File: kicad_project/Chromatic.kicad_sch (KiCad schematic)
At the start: 159 parts, among them J1 J1, J2 J2, U1 ESP32-S3

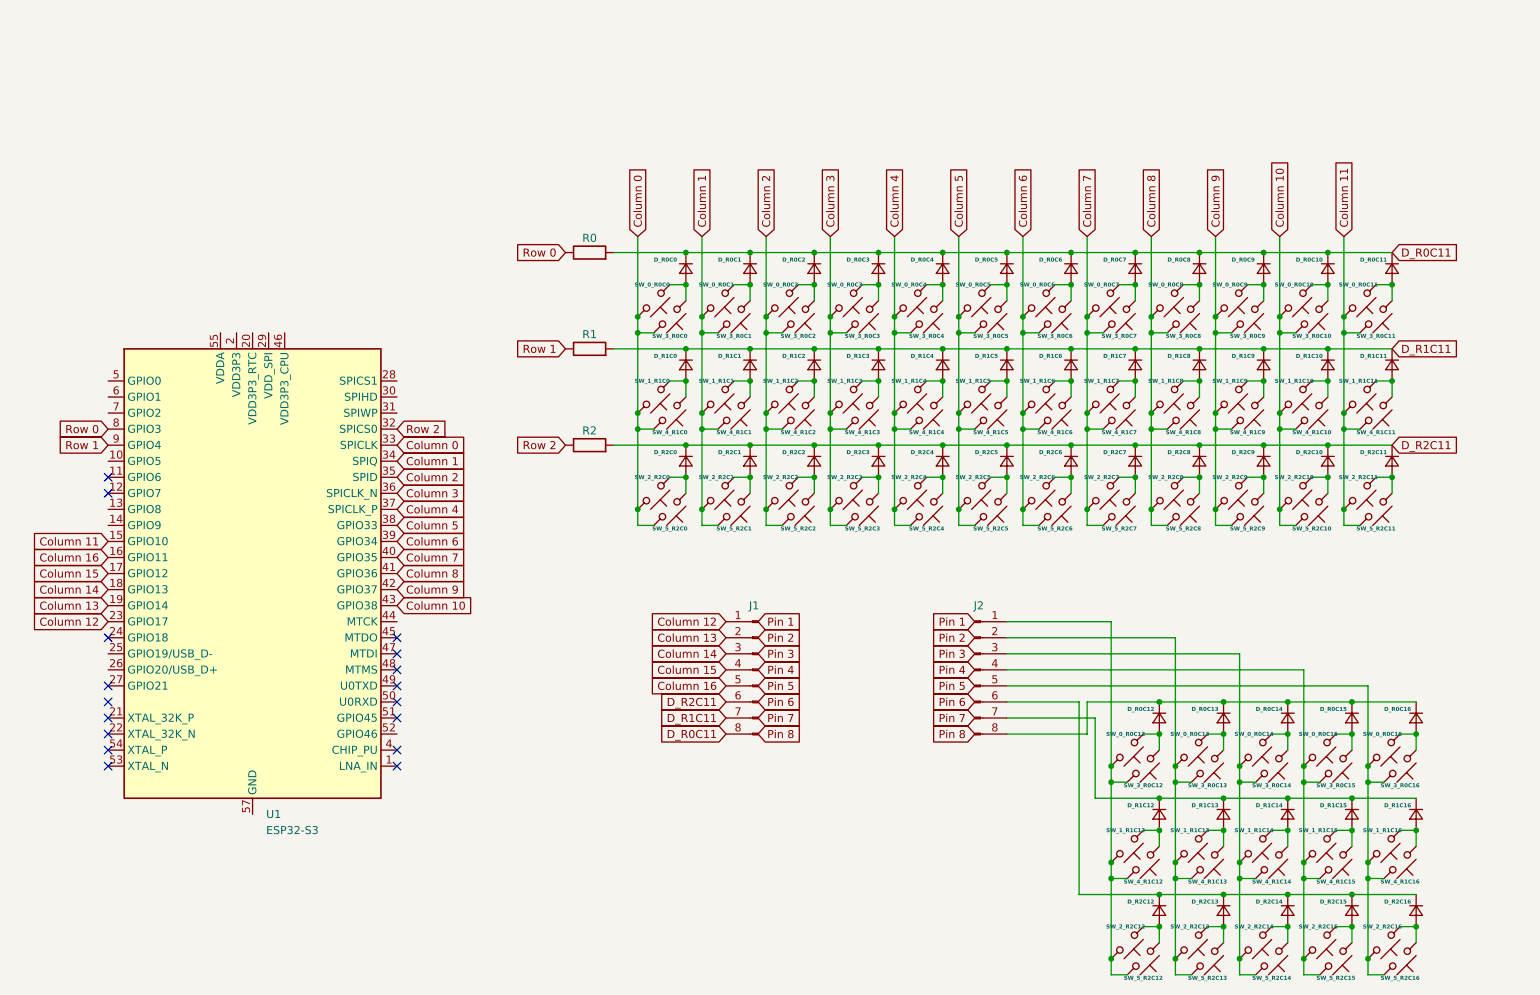
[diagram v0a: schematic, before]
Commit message: arrumado pcb e footprint
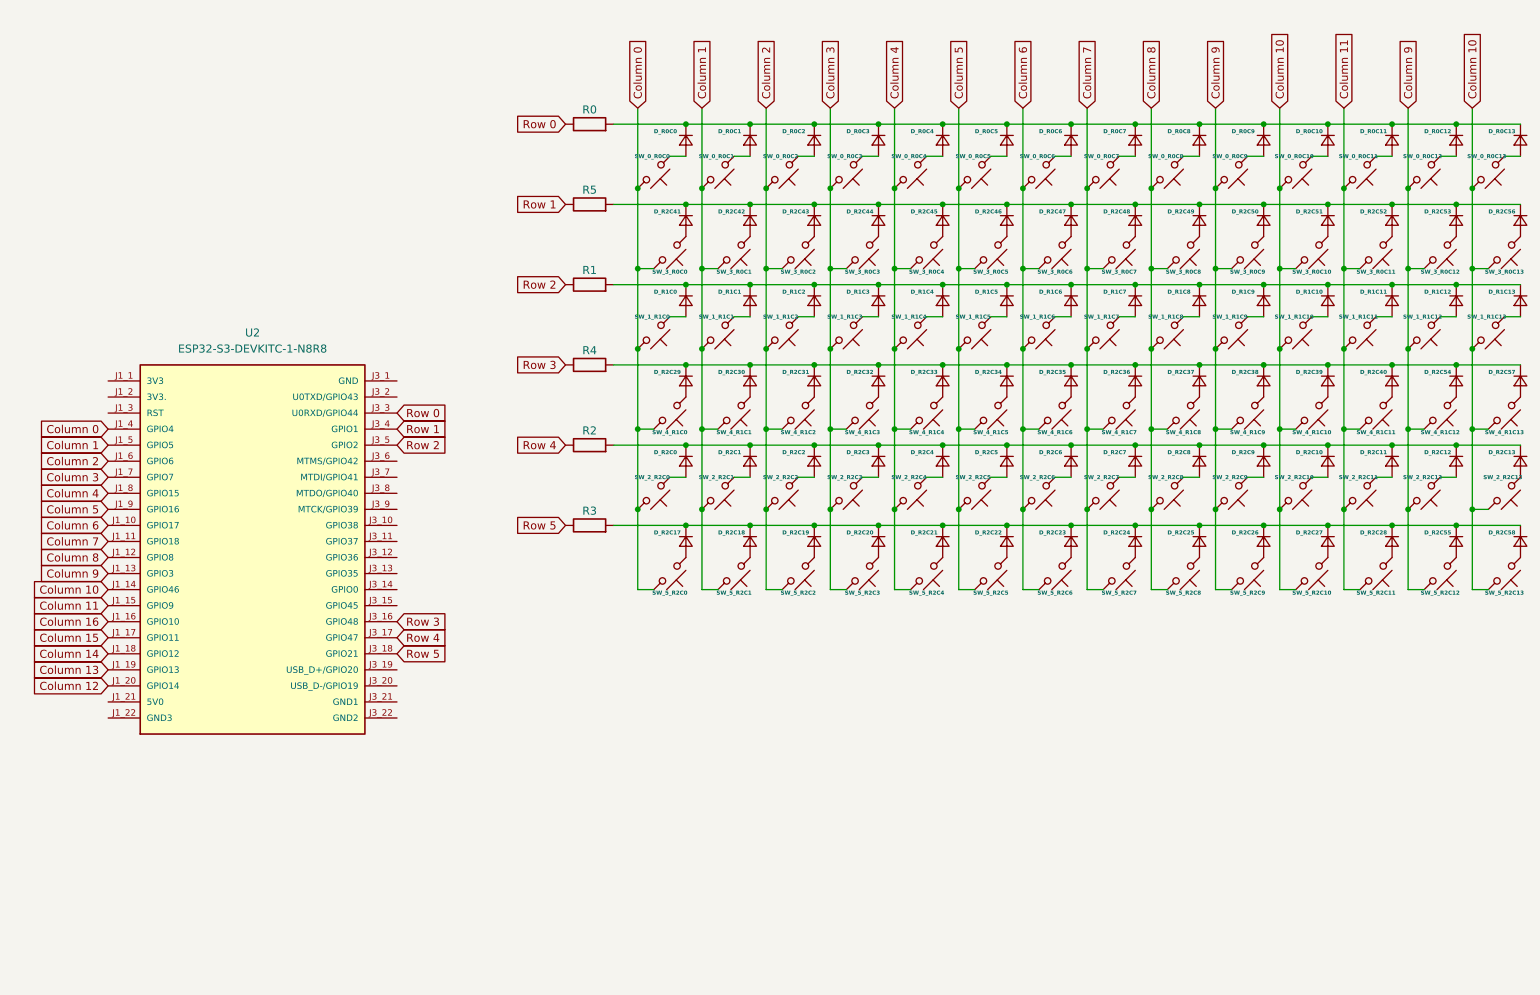
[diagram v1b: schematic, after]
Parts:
- removed D_R0C14, D_R0C15, D_R0C16, D_R1C14, D_R1C15, D_R1C16, D_R2C14, D_R2C15, D_R2C16: (no value), ScottoKeebs_Components:Diode_DO-35, symbol ScottoKeebs:Placeholder_Diode
- removed J1: J1, Connector_PinHeader_2.54mm:PinHeader_1x08_P2.54mm_Vertical, symbol Connector:Conn_01x08_Pin
- removed J2: J2, Connector_PinHeader_2.54mm:PinHeader_1x08_P2.54mm_Vertical, symbol Connector:Conn_01x08_Pin
- removed SW_0_R0C14, SW_0_R0C15, SW_0_R0C16, SW_1_R1C14, SW_1_R1C15, SW_1_R1C16, SW_2_R2C14, SW_2_R2C15, SW_2_R2C16, SW_3_R0C14, SW_3_R0C15, SW_3_R0C16, SW_4_R1C14, SW_4_R1C15, SW_4_R1C16, SW_5_R2C14, SW_5_R2C15, SW_5_R2C16: Keyswitch, ScottoKeebs_Hotswap:Hotswap_MX_1.00u, symbol ScottoKeebs:Placeholder_Keyswitch
- removed U1: ESP32-S3, Module:XCVR_ESP32-S3-DEVKIT-LIPO, symbol MCU_Espressif:ESP32-S3
- added D_R2C17, D_R2C18, D_R2C19, D_R2C20, D_R2C21, D_R2C22, D_R2C23, D_R2C24, D_R2C25, D_R2C26, D_R2C27, D_R2C28, D_R2C29, D_R2C30, D_R2C31, D_R2C32, D_R2C33, D_R2C34, D_R2C35, D_R2C36, D_R2C37, D_R2C38, D_R2C39, D_R2C40, D_R2C41, D_R2C42, D_R2C43, D_R2C44, D_R2C45, D_R2C46, D_R2C47, D_R2C48, D_R2C49, D_R2C50, D_R2C51, D_R2C52, D_R2C53, D_R2C54, D_R2C55, D_R2C56, D_R2C57, D_R2C58: (no value), ScottoKeebs_Components:Diode_DO-35, symbol ScottoKeebs:Placeholder_Diode
- added R3, R4, R5: Resistor, Resistor_THT:R_Axial_DIN0207_L6.3mm_D2.5mm_P7.62mm_Horizontal, symbol ScottoKeebs:Placeholder_Resistor
- added U2: ESP32-S3-DEVKITC-1-N8R8, RF_Module:ESP32-S3-DEVKITC-1-N8R8, symbol ESP32-S3-DEVKITC-1-N8R8:ESP32-S3-DEVKITC-1-N8R8
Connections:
- net D_R0C11 is gone; now on an unnamed net: D_R0C0.1 (K), D_R0C1.1 (K), D_R0C10.1 (K), D_R0C11.1 (K), D_R0C2.1 (K), D_R0C3.1 (K), D_R0C4.1 (K), D_R0C5.1 (K), D_R0C6.1 (K), D_R0C7.1 (K), D_R0C8.1 (K), D_R0C9.1 (K), R0.2
- net D_R1C11 is gone; now on an unnamed net: D_R1C0.1 (K), D_R1C1.1 (K), D_R1C10.1 (K), D_R1C11.1 (K), D_R1C2.1 (K), D_R1C3.1 (K), D_R1C4.1 (K), D_R1C5.1 (K), D_R1C6.1 (K), D_R1C7.1 (K), D_R1C8.1 (K), D_R1C9.1 (K), R1.2
- net D_R2C11 is gone; now on an unnamed net: D_R2C0.1 (K), D_R2C1.1 (K), D_R2C10.1 (K), D_R2C11.1 (K), D_R2C2.1 (K), D_R2C3.1 (K), D_R2C4.1 (K), D_R2C5.1 (K), D_R2C6.1 (K), D_R2C7.1 (K), D_R2C8.1 (K), D_R2C9.1 (K), R2.2
- net Column 0: now also U2.J1_4 (GPIO4)
- net Column 1: now also U2.J1_5 (GPIO5)
- net Column 10: now also SW_0_R0C13.1, SW_1_R1C13.1, SW_2_R2C13.1, SW_3_R0C13.1, SW_4_R1C13.1, SW_5_R2C13.1, U2.J1_14 (GPIO46)
- net Column 11: now also U2.J1_15 (GPIO9)
- net Column 12: now also U2.J1_20 (GPIO14)
- net Column 13: now also U2.J1_19 (GPIO13)
- net Column 14: now also U2.J1_18 (GPIO12)
- net Column 15: now also U2.J1_17 (GPIO11)
- net Column 16: now also U2.J1_16 (GPIO10)
- net Column 2: now also U2.J1_6 (GPIO6)
- net Column 3: now also U2.J1_7 (GPIO7)
- net Column 4: now also U2.J1_8 (GPIO15)
- net Column 5: now also U2.J1_9 (GPIO16)
- net Column 6: now also U2.J1_10 (GPIO17)
- net Column 7: now also U2.J1_11 (GPIO18)
- net Column 8: now also U2.J1_12 (GPIO8)
- net Column 9: now also SW_0_R0C12.1, SW_1_R1C12.1, SW_2_R2C12.1, SW_3_R0C12.1, SW_4_R1C12.1, SW_5_R2C12.1, U2.J1_13 (GPIO3)
- net Row 0: now also U2.J3_3 (U0RXD/GPIO44)
- net Row 1: now also R5.1, U2.J3_4 (GPIO1); no longer R1.1
- net Row 2: now also R1.1, U2.J3_5 (GPIO2); no longer R2.1
- net at D_R1C7.2 (A), SW_1_R1C7.2: no longer SW_4_R1C7.2
- net at D_R0C3.2 (A), SW_0_R0C3.2: no longer SW_3_R0C3.2
- net at D_R2C4.2 (A), SW_2_R2C4.2: no longer SW_5_R2C4.2
- net at D_R1C0.2 (A), SW_1_R1C0.2: no longer SW_4_R1C0.2
- net at D_R2C2.2 (A), SW_2_R2C2.2: no longer SW_5_R2C2.2
- net at D_R0C1.2 (A), SW_0_R0C1.2: no longer SW_3_R0C1.2
- net at D_R1C8.2 (A), SW_1_R1C8.2: no longer SW_4_R1C8.2
- net at D_R1C13.2 (A), SW_1_R1C13.2: no longer SW_4_R1C13.2
- net at D_R2C1.2 (A), SW_2_R2C1.2: no longer SW_5_R2C1.2
- net at D_R2C6.2 (A), SW_2_R2C6.2: no longer SW_5_R2C6.2
- net at D_R2C5.2 (A), SW_2_R2C5.2: no longer SW_5_R2C5.2
- net at D_R1C3.2 (A), SW_1_R1C3.2: no longer SW_4_R1C3.2
- net at D_R2C0.2 (A), SW_2_R2C0.2: no longer SW_5_R2C0.2
- net at D_R1C4.2 (A), SW_1_R1C4.2: no longer SW_4_R1C4.2
- net at D_R2C13.2 (A), SW_2_R2C13.2: no longer SW_5_R2C13.2
- net at D_R0C7.2 (A), SW_0_R0C7.2: no longer SW_3_R0C7.2
- net at D_R0C0.2 (A), SW_0_R0C0.2: no longer SW_3_R0C0.2
- net at D_R1C9.2 (A), SW_1_R1C9.2: no longer SW_4_R1C9.2
- net at D_R1C1.2 (A), SW_1_R1C1.2: no longer SW_4_R1C1.2
- net at D_R0C2.2 (A), SW_0_R0C2.2: no longer SW_3_R0C2.2
- net at D_R1C6.2 (A), SW_1_R1C6.2: no longer SW_4_R1C6.2
- net at D_R0C13.2 (A), SW_0_R0C13.2: no longer SW_3_R0C13.2
- net at D_R0C6.2 (A), SW_0_R0C6.2: no longer SW_3_R0C6.2
- net at D_R0C11.2 (A), SW_0_R0C11.2: no longer SW_3_R0C11.2
- net at D_R1C11.2 (A), SW_1_R1C11.2: no longer SW_4_R1C11.2
- net at D_R1C2.2 (A), SW_1_R1C2.2: no longer SW_4_R1C2.2
- net at D_R2C9.2 (A), SW_2_R2C9.2: no longer SW_5_R2C9.2
- net at D_R2C10.2 (A), SW_2_R2C10.2: no longer SW_5_R2C10.2
- net at D_R2C3.2 (A), SW_2_R2C3.2: no longer SW_5_R2C3.2
- net at D_R1C5.2 (A), SW_1_R1C5.2: no longer SW_4_R1C5.2
- net at D_R0C8.2 (A), SW_0_R0C8.2: no longer SW_3_R0C8.2
- net at D_R2C8.2 (A), SW_2_R2C8.2: no longer SW_5_R2C8.2
- net at D_R0C5.2 (A), SW_0_R0C5.2: no longer SW_3_R0C5.2
- net at D_R0C4.2 (A), SW_0_R0C4.2: no longer SW_3_R0C4.2
- net at D_R2C12.2 (A), SW_2_R2C12.2: no longer SW_5_R2C12.2
- net at D_R2C7.2 (A), SW_2_R2C7.2: no longer SW_5_R2C7.2
- net at D_R0C9.2 (A), SW_0_R0C9.2: no longer SW_3_R0C9.2
- net at D_R0C10.2 (A), SW_0_R0C10.2: no longer SW_3_R0C10.2
- net at D_R2C11.2 (A), SW_2_R2C11.2: no longer SW_5_R2C11.2
- net at D_R1C10.2 (A), SW_1_R1C10.2: no longer SW_4_R1C10.2
- net at D_R1C12.2 (A), SW_1_R1C12.2: no longer SW_4_R1C12.2
- net at D_R0C12.2 (A), SW_0_R0C12.2: no longer SW_3_R0C12.2
- new net: D_R2C44.2 (A), SW_3_R0C3.2
- new net: D_R2C55.2 (A), SW_5_R2C12.2
- new net: D_R2C41.1 (K), D_R2C42.1 (K), D_R2C43.1 (K), D_R2C44.1 (K), D_R2C45.1 (K), D_R2C46.1 (K), D_R2C47.1 (K), D_R2C48.1 (K), D_R2C49.1 (K), D_R2C50.1 (K), D_R2C51.1 (K), D_R2C52.1 (K), D_R2C53.1 (K), D_R2C56.1 (K), R5.2
- new net: D_R2C53.2 (A), SW_3_R0C12.2
- new net: D_R2C17.1 (K), D_R2C18.1 (K), D_R2C19.1 (K), D_R2C20.1 (K), D_R2C21.1 (K), D_R2C22.1 (K), D_R2C23.1 (K), D_R2C24.1 (K), D_R2C25.1 (K), D_R2C26.1 (K), D_R2C27.1 (K), D_R2C28.1 (K), D_R2C55.1 (K), D_R2C58.1 (K), R3.2
- new net: D_R2C50.2 (A), SW_3_R0C9.2
- new net: D_R2C37.2 (A), SW_4_R1C8.2
- new net: D_R2C22.2 (A), SW_5_R2C5.2
- new net: D_R2C56.2 (A), SW_3_R0C13.2
- new net: D_R2C43.2 (A), SW_3_R0C2.2
- new net: D_R2C29.1 (K), D_R2C30.1 (K), D_R2C31.1 (K), D_R2C32.1 (K), D_R2C33.1 (K), D_R2C34.1 (K), D_R2C35.1 (K), D_R2C36.1 (K), D_R2C37.1 (K), D_R2C38.1 (K), D_R2C39.1 (K), D_R2C40.1 (K), D_R2C54.1 (K), D_R2C57.1 (K), R4.2
- new net: D_R2C33.2 (A), SW_4_R1C4.2
- new net: D_R2C38.2 (A), SW_4_R1C9.2
- new net: D_R2C36.2 (A), SW_4_R1C7.2
- new net: D_R2C41.2 (A), SW_3_R0C0.2
- new net: D_R2C23.2 (A), SW_5_R2C6.2
- new net: D_R2C32.2 (A), SW_4_R1C3.2
- new net: D_R2C42.2 (A), SW_3_R0C1.2
- new net: D_R2C52.2 (A), SW_3_R0C11.2
- new net: D_R2C25.2 (A), SW_5_R2C8.2
- new net: D_R2C29.2 (A), SW_4_R1C0.2
- new net: D_R2C34.2 (A), SW_4_R1C5.2
- new net: D_R2C27.2 (A), SW_5_R2C10.2
- new net: D_R2C19.2 (A), SW_5_R2C2.2
- new net: D_R2C31.2 (A), SW_4_R1C2.2
- new net: D_R2C48.2 (A), SW_3_R0C7.2
- new net: D_R2C51.2 (A), SW_3_R0C10.2
- new net: D_R2C49.2 (A), SW_3_R0C8.2
- new net: D_R2C46.2 (A), SW_3_R0C5.2
- new net: D_R2C58.2 (A), SW_5_R2C13.2
- new net: D_R2C17.2 (A), SW_5_R2C0.2
- new net: D_R2C21.2 (A), SW_5_R2C4.2
- new net: D_R2C39.2 (A), SW_4_R1C10.2
- new net: D_R2C18.2 (A), SW_5_R2C1.2
- new net: D_R2C24.2 (A), SW_5_R2C7.2
- new net: D_R2C30.2 (A), SW_4_R1C1.2
- new net: D_R2C47.2 (A), SW_3_R0C6.2
- new net: D_R2C45.2 (A), SW_3_R0C4.2
- new net: D_R2C40.2 (A), SW_4_R1C11.2
- new net: D_R2C57.2 (A), SW_4_R1C13.2
- new net: D_R2C20.2 (A), SW_5_R2C3.2
- new net: D_R2C26.2 (A), SW_5_R2C9.2
- new net: D_R2C54.2 (A), SW_4_R1C12.2
- new net: D_R2C28.2 (A), SW_5_R2C11.2
- new net: D_R2C35.2 (A), SW_4_R1C6.2
- new net Row 3: R4.1, U2.J3_16 (GPIO48)
- new net Row 4: R2.1, U2.J3_17 (GPIO47)
- new net Row 5: R3.1, U2.J3_18 (GPIO21)
- no-connect marks 17 -> 0
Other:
- moved on the sheet: D_R0C0, D_R0C1, D_R0C10, D_R0C11, D_R0C2, D_R0C3, D_R0C4, D_R0C5, D_R0C6, D_R0C7, D_R0C8, D_R0C9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
